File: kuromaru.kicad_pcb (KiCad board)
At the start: 2 copper layers, 126.1 x 97 mm, 63 parts, among them J1 USB_C_Receptacle_USB2.0, J102 Serial, J5 Conn_01x02, SW1 SW_Push, SW2 SW_Push, U1 RP2040, U2 GD25Q80CEIGR, U3 XC6210B332MR-G, U4 25LCxxx, Y1 Crystal_GND24

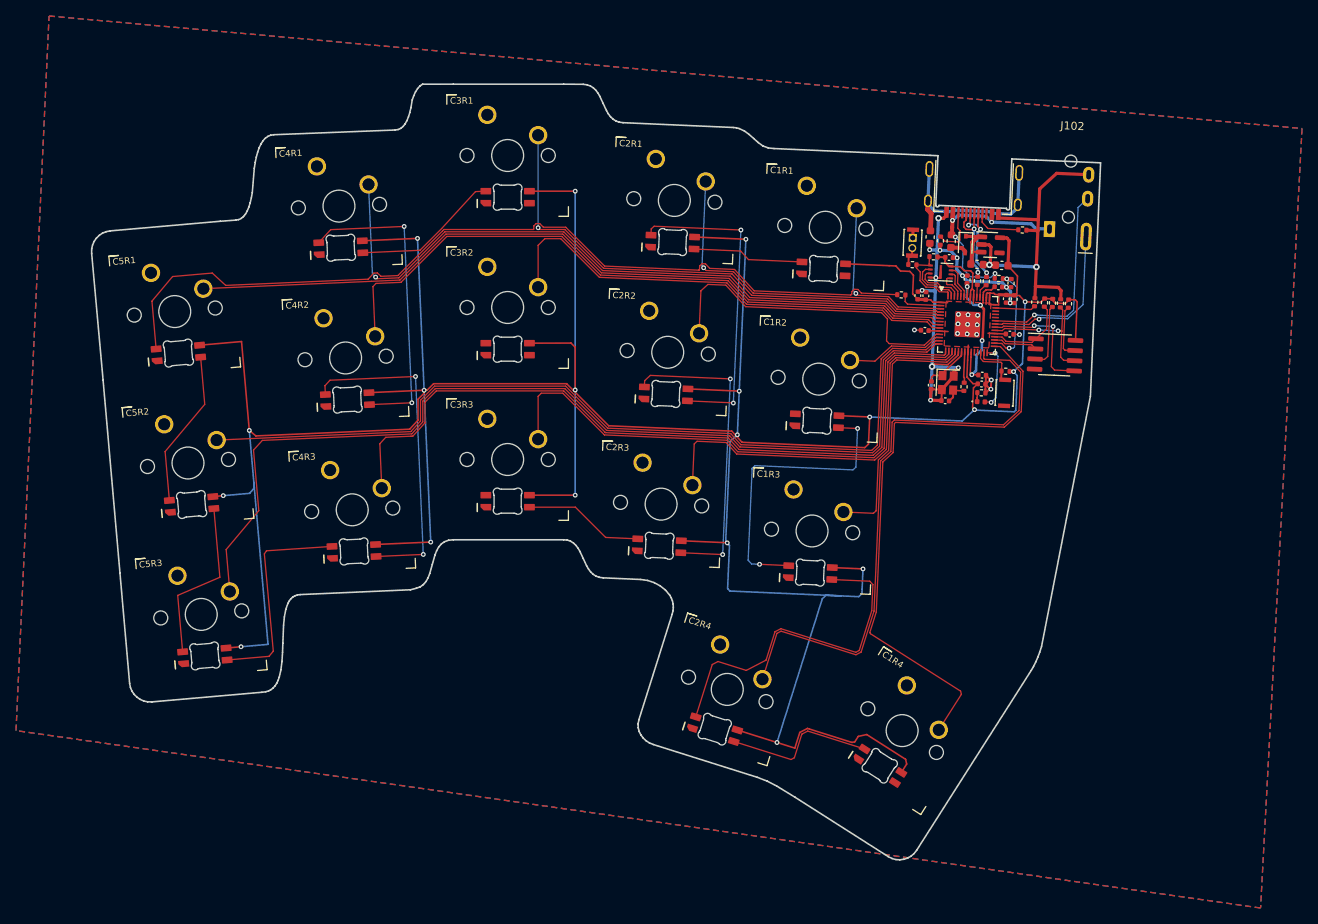
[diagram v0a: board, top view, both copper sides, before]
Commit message: Remove RGB
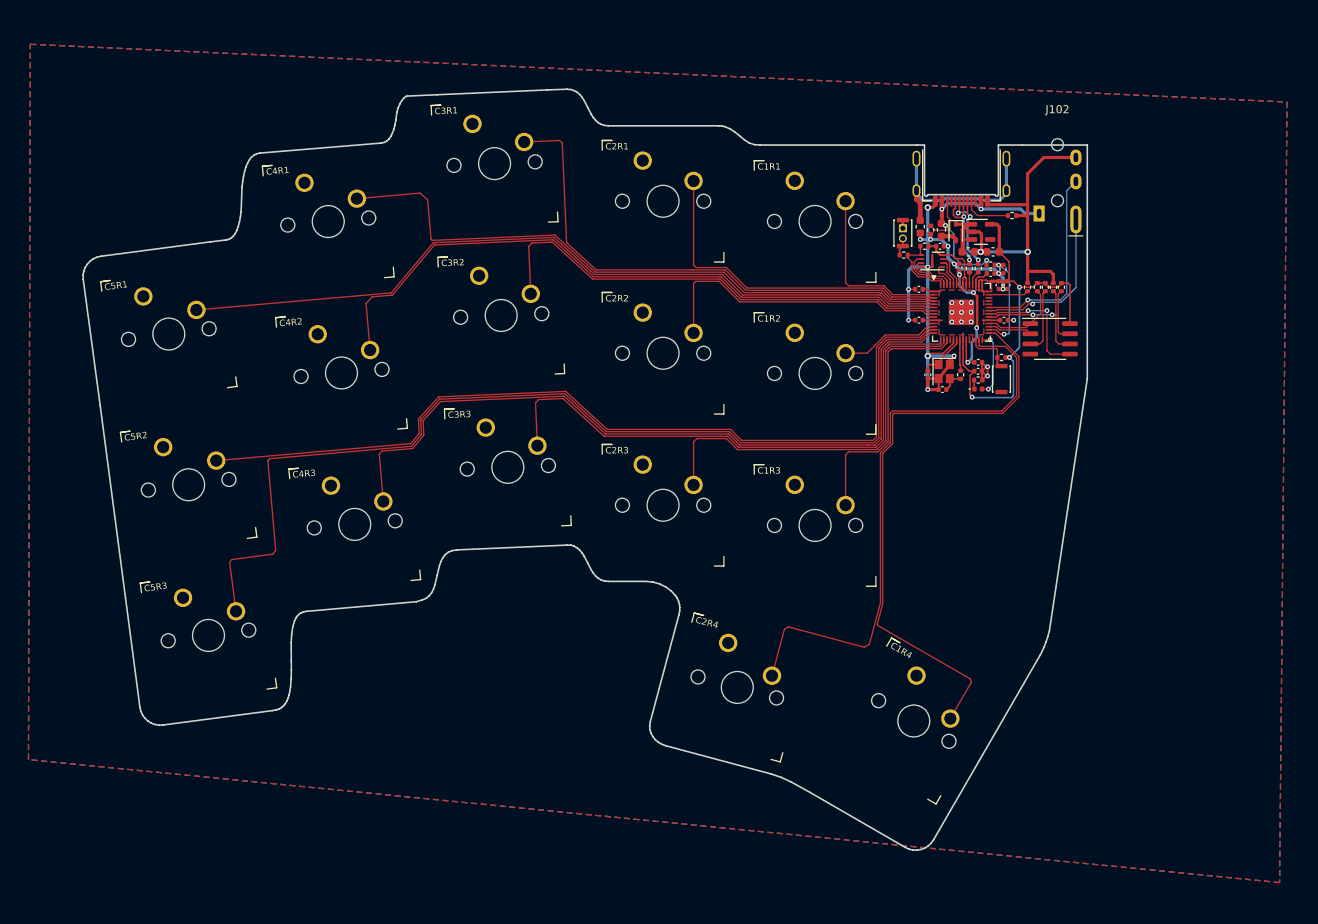
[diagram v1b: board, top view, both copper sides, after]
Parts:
- removed C15: 1µ, Capacitor_SMD:C_0402_1005Metric
- removed R15: 300, Resistor_SMD:R_0402_1005Metric
- C1R1, C1R2, C1R3, C1R4, C2R1, C2R2, C2R3, C2R4, C3R1, C3R2, C3R3, C4R1, C4R2, C4R3, C5R1, C5R2, C5R3: footprint local-libraries:delay_SW_MX_RGB -> local-libraries:delay_SW_MX_flipped
- moved C5R1 2.91 mm to (43.1, 51.6), turned to 7.5 degrees
- moved C5R3 2.78 mm to (48.0, 89.3), turned to 7.5 degrees
- moved C5R2 2.72 mm to (45.5, 70.5), turned to 7.5 degrees
- moved J102 2.55 mm to (154.2, 31.4), turned to 0 degrees
- moved C4R1 2.35 mm to (63.0, 37.6), turned to 5 degrees
- moved J1 2.29 mm to (142.1, 27.6), turned to 180 degrees
- moved R16 2.24 mm to (154.6, 45.8), turned to 90 degrees
- moved R4 2.21 mm to (148.5, 36.8), turned to 180 degrees
- moved R13 2.20 mm to (153.6, 45.8), turned to -90 degrees
- moved R17 2.17 mm to (152.6, 45.8), turned to 90 degrees
- moved R12 2.13 mm to (151.6, 45.8), turned to 90 degrees
- moved U4 2.08 mm to (153.2, 52.2), turned to 0 degrees
- moved R14 2.08 mm to (150.4, 45.8), turned to 90 degrees
- moved U3 2.02 mm to (144.6, 38.8), turned to 0 degrees
- moved C2 2.01 mm to (146.1, 41.3), turned to 180 degrees
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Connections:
- C1R1 pad 1: +3V3 -> GND
- C1R1 pad 2: Net-(C1R1-Pad2) -> switch_c1r1
- C1R2 pad 1: +3V3 -> GND
- C1R2 pad 2: Net-(C1R2-Pad2) -> switch_c1r2
- C1R3 pad 1: +3V3 -> GND
- C1R3 pad 2: Net-(C1R3-Pad2) -> switch_c1r3
- C1R4 pad 1: +3V3 -> GND
- C1R4 pad 2: unconnected-(C1R4-Pad2) -> switch_c1r4
- C2R1 pad 1: +3V3 -> GND
- C2R1 pad 2: Net-(C1R1-Pad4) -> switch_c2r1
- C2R2 pad 1: +3V3 -> GND
- C2R2 pad 2: Net-(C2R1-Pad4) -> switch_c2r2
- C2R3 pad 1: +3V3 -> GND
- C2R3 pad 2: Net-(C2R2-Pad4) -> switch_c2r3
- C2R4 pad 1: +3V3 -> GND
- C2R4 pad 2: Net-(C1R4-Pad4) -> switch_c2r4
- C3R1 pad 1: +3V3 -> GND
- C3R1 pad 2: Net-(C3R1-Pad2) -> switch_c3r1
- C3R2 pad 1: +3V3 -> GND
- C3R2 pad 2: Net-(C3R2-Pad2) -> switch_c3r2
- C3R3 pad 1: +3V3 -> GND
- C3R3 pad 2: Net-(C2R3-Pad4) -> switch_c3r3
- C4R1 pad 1: +3V3 -> GND
- C4R1 pad 2: Net-(C3R1-Pad4) -> switch_c4r1
- C4R2 pad 1: +3V3 -> GND
- C4R2 pad 2: Net-(C4R1-Pad4) -> switch_c4r2
- C4R3 pad 1: +3V3 -> GND
- C4R3 pad 2: Net-(C4R2-Pad4) -> switch_c4r3
- C5R1 pad 1: +3V3 -> GND
- C5R1 pad 2: Net-(C5R1-Pad2) -> switch_c5r1
- C5R2 pad 1: +3V3 -> GND
- C5R2 pad 2: Net-(C5R2-Pad2) -> switch_c5r2
- C5R3 pad 1: +3V3 -> GND
- C5R3 pad 2: Net-(C4R3-Pad4) -> switch_c5r3
- U1 pad 11: switch_c2r2 -> switch_c1r2
- U1 pad 12: switch_c1r2 -> switch_c5r2
- U1 pad 13: switch_c5r2 -> switch_c5r3
- U1 pad 14: switch_c5r3 -> switch_c4r3
- U1 pad 15: switch_c4r3 -> switch_c3r3
- U1 pad 16: switch_c3r3 -> switch_c2r3
- U1 pad 17: switch_c2r3 -> switch_c1r3
- U1 pad 18: switch_c1r3 -> /GPIO15
- U1 pad 2: rgb_din -> switch_c1r1
- U1 pad 3: switch_c1r1 -> switch_c2r1
- U1 pad 4: switch_c2r1 -> switch_c3r1
- U1 pad 5: switch_c3r1 -> switch_c4r1
- U1 pad 6: switch_c4r1 -> switch_c5r1
- U1 pad 7: switch_c5r1 -> switch_c4r2
- U1 pad 8: switch_c4r2 -> switch_c3r2
- U1 pad 9: switch_c3r2 -> switch_c2r2
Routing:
- net +3V3: track 507.6 -> 79.2 mm, vias 19 -> 3
- net Net-(C5R1-Pad4): track 109.6 -> 0.00 mm
- net Net-(C1R3-Pad2): track 42.8 -> 0.00 mm
- net Net-(C4R2-Pad4): track 40.9 -> 0.00 mm, vias 2 -> 0
- net Net-(C2R1-Pad4): track 39.5 -> 0.00 mm, vias 2 -> 0
- net Net-(C2R2-Pad4): track 39.0 -> 0.00 mm, vias 2 -> 0
- net Net-(C4R1-Pad4): track 38.8 -> 0.00 mm, vias 2 -> 0
- net Net-(C1R2-Pad2): track 37.3 -> 0.00 mm, vias 2 -> 0
- net Net-(C4R3-Pad4): track 27.0 -> 0.00 mm
- net Net-(C5R2-Pad2): track 21.4 -> 0.00 mm
- net Net-(C5R1-Pad2): track 19.8 -> 0.00 mm
- net Net-(C1R4-Pad4): track 19.4 -> 0.00 mm
- net Net-(C3R1-Pad4): track 18.5 -> 0.00 mm
- net Net-(C2R3-Pad4): track 15.1 -> 0.00 mm
- net Net-(C1R1-Pad4): track 14.0 -> 0.00 mm
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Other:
- board size 126.1 x 97 mm -> 125.5 x 95.1 mm
